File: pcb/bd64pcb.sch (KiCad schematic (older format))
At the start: 239 parts, among them J1 USB_C_Receptacle_USB2.0, J2 USB_B_Micro, SW1 SW_Push, U1 ATmega32U4-MU, U2 MCP23017_ML, U3 IS31FL3733-QF, Y1 16MHz

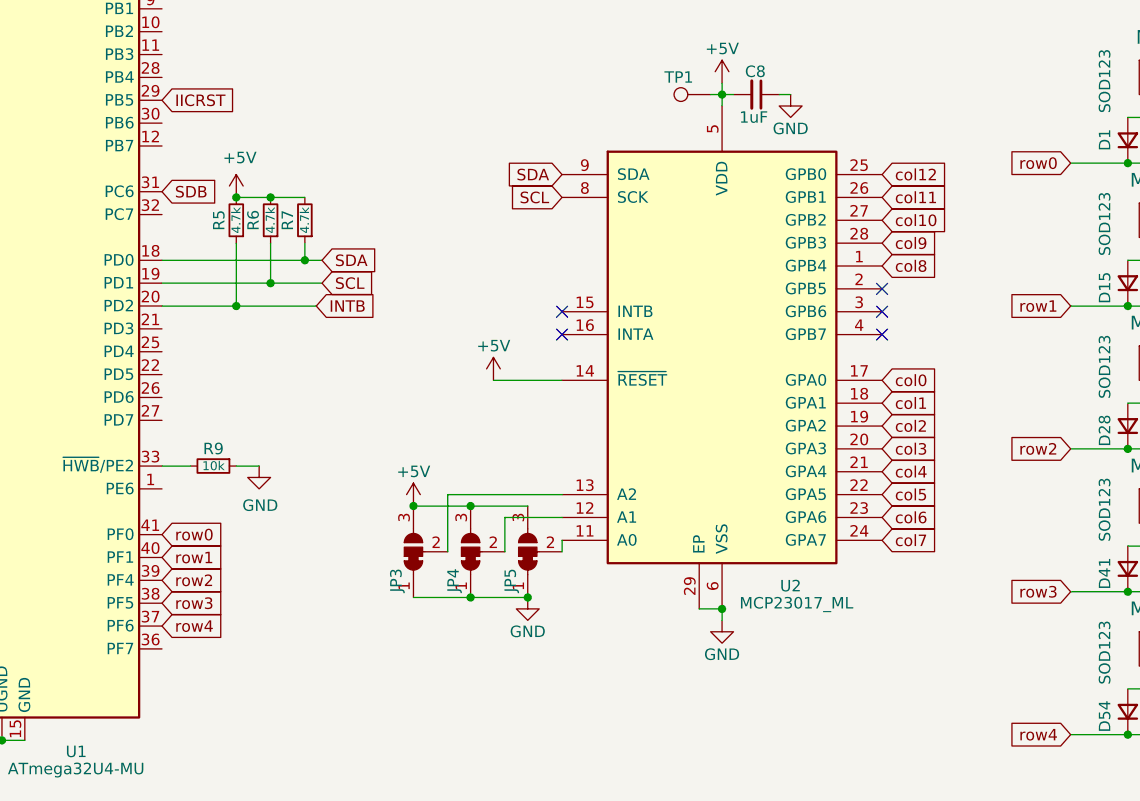
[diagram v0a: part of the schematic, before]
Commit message: no good traces yet
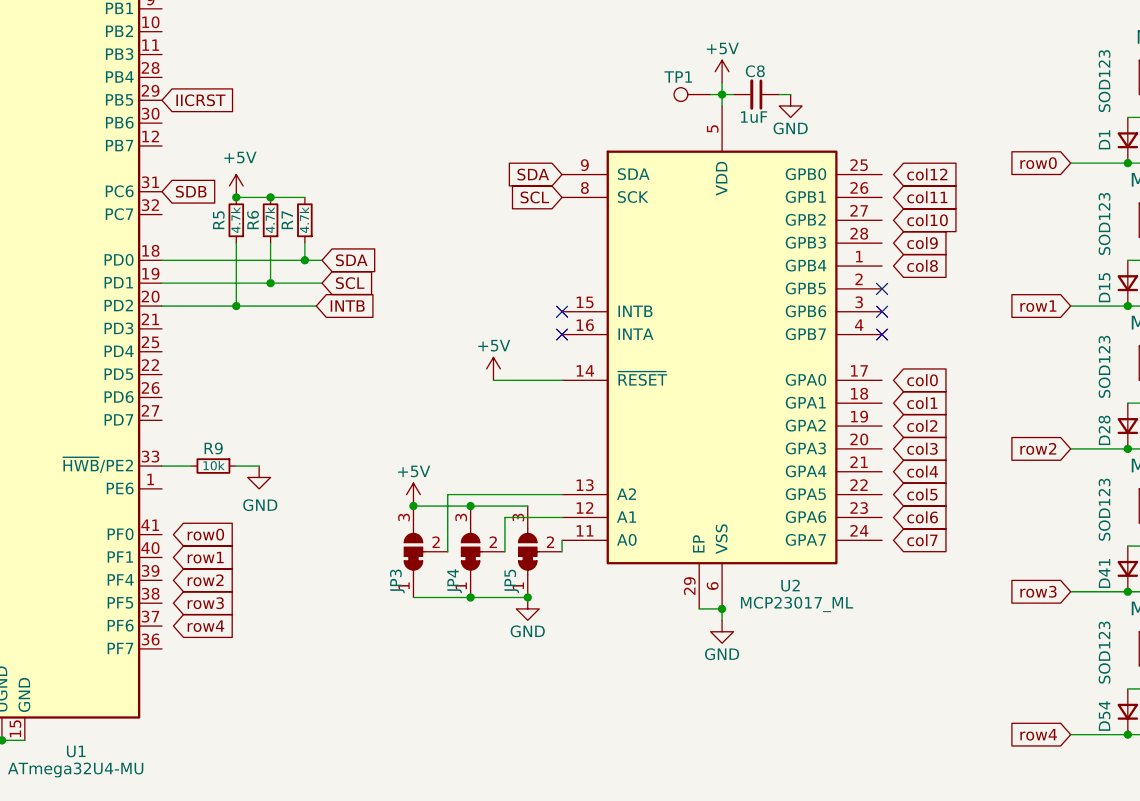
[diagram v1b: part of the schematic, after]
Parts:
- MX1: footprint MX_Alps_Hybrid:MX-1U-NoLED -> MX_Only:MXOnly-1U-NoLED
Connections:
- net col0: no longer U2.17 (GPA0)
- net col1: no longer U2.18 (GPA1)
- net col10: no longer U2.27 (GPB2)
- net col11: no longer U2.26 (GPB1)
- net col12: no longer U2.25 (GPB0)
- net col2: no longer U2.19 (GPA2)
- net col3: no longer U2.20 (GPA3)
- net col4: no longer U2.21 (GPA4)
- net col5: no longer U2.22 (GPA5)
- net col6: no longer U2.23 (GPA6)
- net col7: no longer U2.24 (GPA7)
- net col8: no longer U2.1 (GPB4)
- net col9: no longer U2.28 (GPB3)
- net row0: no longer U1.41 (PF0)
- net row1: no longer U1.40 (PF1)
- net row2: no longer U1.39 (PF4)
- net row3: no longer U1.38 (PF5)
- net row4: no longer U1.37 (PF6)
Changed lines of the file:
@@
 	0    1    1    0
 $EndComp
-Text GLabel 4850 4000 2    50   Input ~ 0
+Text GLabel 4900 4000 2    50   Input ~ 0
 row0
-Text GLabel 4850 4100 2    50   Input ~ 0
+Text GLabel 4900 4100 2    50   Input ~ 0
 row1
-Text GLabel 4850 4200 2    50   Input ~ 0
+Text GLabel 4900 4200 2    50   Input ~ 0
 row2
-Text GLabel 4850 4300 2    50   Input ~ 0
+Text GLabel 4900 4300 2    50   Input ~ 0
 row3
-Text GLabel 4850 4400 2    50   Input ~ 0
+Text GLabel 4900 4400 2    50   Input ~ 0
 row4
 Text GLabel 4525 6750 0    50   Input ~ 0
@@
 SDA
 NoConn ~ 6600 3125
-Text GLabel 8000 3325 2    50   Input ~ 0
+Text GLabel 8050 3325 2    50   Input ~ 0
 col0
-Text GLabel 8000 3425 2    50   Input ~ 0
+Text GLabel 8050 3425 2    50   Input ~ 0
 col1
-Text GLabel 8000 3525 2    50   Input ~ 0
+Text GLabel 8050 3525 2    50   Input ~ 0
 col2
-Text GLabel 8000 3625 2    50   Input ~ 0
+Text GLabel 8050 3625 2    50   Input ~ 0
 col3
-Text GLabel 8000 3725 2    50   Input ~ 0
+Text GLabel 8050 3725 2    50   Input ~ 0
 col4
-Text GLabel 8000 3825 2    50   Input ~ 0
+Text GLabel 8050 3825 2    50   Input ~ 0
 col5
-Text GLabel 8000 3925 2    50   Input ~ 0
+Text GLabel 8050 3925 2    50   Input ~ 0
 col6
-Text GLabel 8000 4025 2    50   Input ~ 0
+Text GLabel 8050 4025 2    50   Input ~ 0
 col7
-Text GLabel 8000 2825 2    50   Input ~ 0
+Text GLabel 8050 2825 2    50   Input ~ 0
 col8
-Text GLabel 8000 2725 2    50   Input ~ 0
+Text GLabel 8050 2725 2    50   Input ~ 0
 col9
-Text GLabel 8000 2625 2    50   Input ~ 0
+Text GLabel 8050 2625 2    50   Input ~ 0
 col10
-Text GLabel 8000 2525 2    50   Input ~ 0
+Text GLabel 8050 2525 2    50   Input ~ 0
 col11
-Text GLabel 8000 2425 2    50   Input ~ 0
+Text GLabel 8050 2425 2    50   Input ~ 0
 col12
 $Comp
@@
 F 0 "MX1" H 9200 2225 60  0000 C CNN
 F 1 "MX-NoLED" H 9200 2150 20  0000 C CNN
-F 2 "MX_Alps_Hybrid:MX-1U-NoLED" H 8600 2000 60  0001 C CNN
+F 2 "MX_Only:MXOnly-1U-NoLED" H 8600 2000 60  0001 C CNN
 F 3 "" H 8600 2000 60  0001 C CNN
 	1    9225 2025

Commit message: boring switch traces
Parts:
- MX2, MX3: footprint MX_Alps_Hybrid:MX-1U-NoLED -> MX_Only:MXOnly-1U-NoLED
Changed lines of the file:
@@
 F 0 "MX3" H 10450 2225 60  0000 C CNN
 F 1 "MX-NoLED" H 10450 2150 20  0000 C CNN
-F 2 "MX_Alps_Hybrid:MX-1U-NoLED" H 9850 2000 60  0001 C CNN
+F 2 "MX_Only:MXOnly-1U-NoLED" H 9850 2000 60  0001 C CNN
 F 3 "" H 9850 2000 60  0001 C CNN
 	1    10475 2025
@@
 F 0 "MX2" H 9825 2225 60  0000 C CNN
 F 1 "MX-NoLED" H 9825 2150 20  0000 C CNN
-F 2 "MX_Alps_Hybrid:MX-1U-NoLED" H 9225 2000 60  0001 C CNN
+F 2 "MX_Only:MXOnly-1U-NoLED" H 9225 2000 60  0001 C CNN
 F 3 "" H 9225 2000 60  0001 C CNN
 	1    9850 2025
